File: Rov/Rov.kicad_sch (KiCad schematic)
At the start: 1 part, among them Q1 IRLZ44N

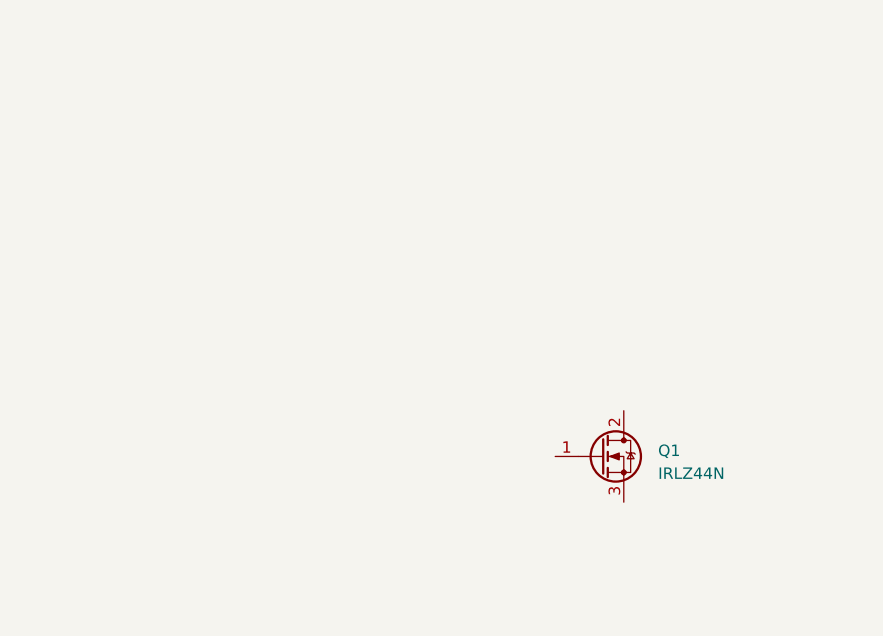
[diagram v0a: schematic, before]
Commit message: Learning kicad
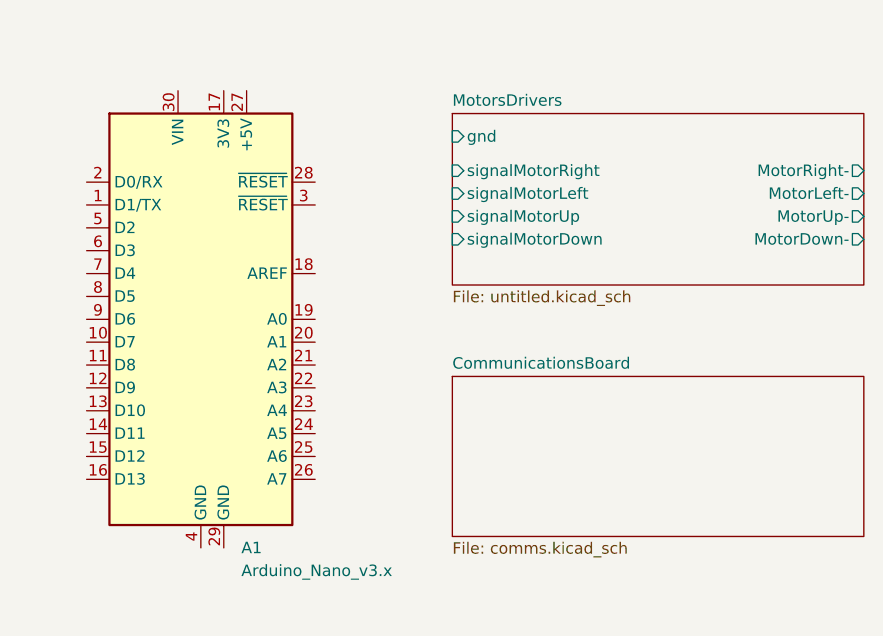
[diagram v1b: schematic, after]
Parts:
- removed Q1: IRLZ44N, Package_TO_SOT_THT:TO-220-3_Vertical, symbol Transistor_FET:IRLZ44N
- added A1: Arduino_Nano_v3.x, Module:Arduino_Nano, symbol MCU_Module:Arduino_Nano_v3.x
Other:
- added sheet CommunicationsBoard (comms.kicad_sch)
- added sheet MotorsDrivers (untitled.kicad_sch)
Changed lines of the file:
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@@
 (kicad_sch (version 20230121) (generator eeschema)
   (paper "A4")
-  (symbol (lib_id "Transistor_FET:IRLZ44N") (at 120.65 90.17 0) (unit 1)
+  (symbol (lib_id "MCU_Module:Arduino_Nano_v3.x") (at 76.2 74.93 0) (unit 1)
     (in_bom yes) (on_board yes) (dnp no) (fields_autoplaced)
-    (property "Reference" "Q1" (at 127 89.535 0)
+    (property "Reference" "A1" (at 80.6959 100.33 0)
       (effects (font (size 1.27 1.27)) (justify left))
     )
-    (property "Value" "IRLZ44N" (at 127 92.075 0)
+    (property "Value" "Arduino_Nano_v3.x" (at 80.6959 102.87 0)
       (effects (font (size 1.27 1.27)) (justify left))
     )
-    (property "Footprint" "Package_TO_SOT_THT:TO-220-3_Vertical" (at 127 92.075 0)
-      (effects (font (size 1.27 1.27) italic) (justify left) hide)
+    (property "Footprint" "Module:Arduino_Nano" (at 76.2 74.93 0)
+      (effects (font (size 1.27 1.27) italic) hide)
     )
-    (property "Datasheet" "http://www.irf.com/product-info/datasheets/data/irlz44n.pdf" (at 120.65 90.17 0)
-      (effects (font (size 1.27 1.27)) (justify left) hide)
+    (property "Datasheet" "http://www.mouser.com/pdfdocs/Gravitech_Arduino_Nano3_0.pdf" (at 76.2 74.93 0)
+      (effects (font (size 1.27 1.27)) hide)
     )
     (pin "1")
+    (pin "10")
+    (pin "11")
+    (pin "12")
+    (pin "13")
+    (pin "14")
+    (pin "15")
+    (pin "16")
+    (pin "17")
+    (pin "18")
+    (pin "19")
     (pin "2")
+    (pin "20")
+    (pin "21")
+    (pin "22")
+    (pin "23")
+    (pin "24")
+    (pin "25")
+    (pin "26")
+    (pin "27")
+    (pin "28")
+    (pin "29")
     (pin "3")
+    (pin "30")
+    (pin "4")
+    (pin "5")
+    (pin "6")
+    (pin "7")
+    (pin "8")
+    (pin "9")
     (instances
       (project "Rov"
         (path "/195799e7-2545-43ed-8a08-3008b09b45b7"
-          (reference "Q1") (unit 1)
+          (reference "A1") (unit 1)
         )
       )
     )
+  )
+  (sheet (at 104.14 81.28) (size 45.72 17.78) (fields_autoplaced)
+    (stroke (width 0.1524) (type solid))
+    (fill (color 0 0 0 0.0000))
+    (property "Sheetname" "CommunicationsBoard" (at 104.14 80.5684 0)
+      (effects (font (size 1.27 1.27)) (justify left bottom))
+    )
+    (property "Sheetfile" "comms.kicad_sch" (at 104.14 99.6446 0)
+      (effects (font (size 1.27 1.27)) (justify left top))
+    )
+    (instances
+      (project "Rov"
+        (path "/195799e7-2545-43ed-8a08-3008b09b45b7" (page "3"))
+      )
+    )
+  )
+  (sheet (at 104.14 52.07) (size 45.72 19.05) (fields_autoplaced)
+    (stroke (width 0.1524) (type solid))
+    (fill (color 0 0 0 0.0000))
+    (property "Sheetname" "MotorsDrivers" (at 104.14 51.3584 0)
+      (effects (font (size 1.27 1.27)) (justify left bottom))
+    )
+    (property "Sheetfile" "untitled.kicad_sch" (at 104.14 71.7046 0)
+      (effects (font (size 1.27 1.27)) (justify left top))
+    )
+    (pin "MotorRight-" output (at 149.86 58.42 0)
+      (effects (font (size 1.27 1.27)) (justify right))
+    )
+    (pin "MotorDown-" output (at 149.86 66.04 0)
+      (effects (font (size 1.27 1.27)) (justify right))
+    )
+    (pin "MotorUp-" output (at 149.86 63.5 0)
+      (effects (font (size 1.27 1.27)) (justify right))
+    )
+    (pin "MotorLeft-" output (at 149.86 60.96 0)
+      (effects (font (size 1.27 1.27)) (justify right))
+    )
+    (pin "gnd" input (at 104.14 54.61 180)
+      (effects (font (size 1.27 1.27)) (justify left))
+    )
+    (pin "signalMotorRight" input (at 104.14 58.42 180)
+      (effects (font (size 1.27 1.27)) (justify left))
+    )
+    (pin "signalMotorLeft" input (at 104.14 60.96 180)
+      (effects (font (size 1.27 1.27)) (justify left))
+    )
+    (pin "signalMotorUp" input (at 104.14 63.5 180)
+      (effects (font (size 1.27 1.27)) (justify left))
+    )
+    (pin "signalMotorDown" input (at 104.14 66.04 180)
+      (effects (font (size 1.27 1.27)) (justify left))
+    )
+    (instances
+      (project "Rov"
+        (path "/195799e7-2545-43ed-8a08-3008b09b45b7" (page "2"))
+      )
+    )

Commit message: Added more wiring
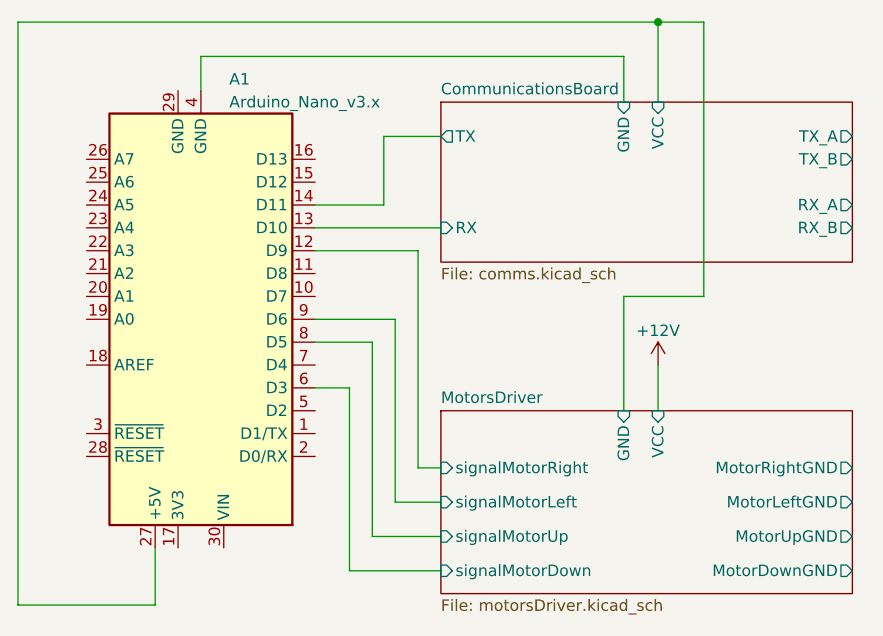
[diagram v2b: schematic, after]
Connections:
- net MotorsDriver/signalMotorRight: now reaches A1.12 (D9)
- net CommunicationsBoard/RX: now reaches A1.13 (D10)
- net CommunicationsBoard/TX: now reaches A1.14 (D11)
- net CommunicationsBoard/VCC: now reaches A1.27 (+5V)
- net CommunicationsBoard/GND: now reaches A1.4 (GND)
- net MotorsDriver/signalMotorDown: now reaches A1.6 (D3)
- net MotorsDriver/signalMotorUp: now reaches A1.8 (D5)
- net MotorsDriver/signalMotorLeft: now reaches A1.9 (D6)
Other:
- removed sheet MotorsDrivers
- added sheet MotorsDriver (motorsDriver.kicad_sch)
- sheet CommunicationsBoard ports: added GND, RX, RX_A, RX_B, TX, TX_A, TX_B, VCC; removed none
- moved on the sheet: A1
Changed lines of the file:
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@@
 (kicad_sch (version 20230121) (generator eeschema)
   (paper "A4")
-  (symbol (lib_id "MCU_Module:Arduino_Nano_v3.x") (at 76.2 74.93 0) (unit 1)
+  (junction (at 127 41.91) (diameter 0) (color 0 0 0 0)
+  )
+  (wire (pts (xy 95.25 99.06) (xy 95.25 77.47))
+    (stroke (width 0) (type default))
+  )
+  (wire (pts (xy 96.52 54.61) (xy 102.87 54.61))
+    (stroke (width 0) (type default))
+  )
+  (wire (pts (xy 102.87 91.44) (xy 100.33 91.44))
+    (stroke (width 0) (type default))
+  )
+  (wire (pts (xy 132.08 72.39) (xy 132.08 41.91))
+    (stroke (width 0) (type default))
+  )
+  (wire (pts (xy 76.2 45.72) (xy 123.19 45.72))
+    (stroke (width 0) (type default))
+  )
+  (wire (pts (xy 96.52 54.61) (xy 96.52 62.23))
+    (stroke (width 0) (type default))
+  )
+  (wire (pts (xy 97.79 95.25) (xy 102.87 95.25))
+    (stroke (width 0) (type default))
+  )
+  (wire (pts (xy 55.88 41.91) (xy 55.88 106.68))
+    (stroke (width 0) (type default))
+  )
+  (wire (pts (xy 132.08 41.91) (xy 127 41.91))
+    (stroke (width 0) (type default))
+  )
+  (wire (pts (xy 92.71 102.87) (xy 102.87 102.87))
+    (stroke (width 0) (type default))
+  )
+  (wire (pts (xy 123.19 45.72) (xy 123.19 50.8))
+    (stroke (width 0) (type default))
+  )
+  (wire (pts (xy 76.2 49.53) (xy 76.2 45.72))
+    (stroke (width 0) (type default))
+  )
+  (wire (pts (xy 123.19 85.09) (xy 123.19 72.39))
+    (stroke (width 0) (type default))
+  )
+  (wire (pts (xy 127 41.91) (xy 55.88 41.91))
+    (stroke (width 0) (type default))
+  )
+  (wire (pts (xy 100.33 67.31) (xy 88.9 67.31))
+    (stroke (width 0) (type default))
+  )
+  (wire (pts (xy 92.71 82.55) (xy 92.71 102.87))
+    (stroke (width 0) (type default))
+  )
+  (wire (pts (xy 88.9 74.93) (xy 97.79 74.93))
+    (stroke (width 0) (type default))
+  )
+  (wire (pts (xy 88.9 82.55) (xy 92.71 82.55))
+    (stroke (width 0) (type default))
+  )
+  (wire (pts (xy 88.9 77.47) (xy 95.25 77.47))
+    (stroke (width 0) (type default))
+  )
+  (wire (pts (xy 127 50.8) (xy 127 41.91))
+    (stroke (width 0) (type default))
+  )
+  (wire (pts (xy 88.9 62.23) (xy 96.52 62.23))
+    (stroke (width 0) (type default))
+  )
+  (wire (pts (xy 102.87 99.06) (xy 95.25 99.06))
+    (stroke (width 0) (type default))
+  )
+  (wire (pts (xy 127 80.01) (xy 127 85.09))
+    (stroke (width 0) (type default))
+  )
+  (wire (pts (xy 71.12 106.68) (xy 71.12 100.33))
+    (stroke (width 0) (type default))
+  )
+  (wire (pts (xy 55.88 106.68) (xy 71.12 106.68))
+    (stroke (width 0) (type default))
+  )
+  (wire (pts (xy 88.9 64.77) (xy 102.87 64.77))
+    (stroke (width 0) (type default))
+  )
+  (wire (pts (xy 97.79 74.93) (xy 97.79 95.25))
+    (stroke (width 0) (type default))
+  )
+  (wire (pts (xy 100.33 91.44) (xy 100.33 67.31))
+    (stroke (width 0) (type default))
+  )
+  (wire (pts (xy 123.19 72.39) (xy 132.08 72.39))
+    (stroke (width 0) (type default))
+  )
+  (symbol (lib_id "power:+12V") (at 127 80.01 0) (unit 1)
     (in_bom yes) (on_board yes) (dnp no) (fields_autoplaced)
-    (property "Reference" "A1" (at 80.6959 100.33 0)
-      (effects (font (size 1.27 1.27)) (justify left))
-    )
-    (property "Value" "Arduino_Nano_v3.x" (at 80.6959 102.87 0)
-      (effects (font (size 1.27 1.27)) (justify left))
+    (property "Reference" "#PWR01" (at 127 83.82 0)
+      (effects (font (size 1.27 1.27)) hide)
+    )
+    (property "Value" "+12V" (at 127 76.2 0)
+      (effects (font (size 1.27 1.27)))
+    )
+    (property "Footprint" "" (at 127 80.01 0)
+      (effects (font (size 1.27 1.27)) hide)
+    )
+    (property "Datasheet" "" (at 127 80.01 0)
+      (effects (font (size 1.27 1.27)) hide)
+    )
+    (pin "1")
+    (instances
+      (project "Rov"
+        (path "/195799e7-2545-43ed-8a08-3008b09b45b7"
+          (reference "#PWR01") (unit 1)
+        )
+      )
+    )
+  )
+  (symbol (lib_id "MCU_Module:Arduino_Nano_v3.x") (at 76.2 74.93 180) (unit 1)
+    (in_bom yes) (on_board yes) (dnp no) (fields_autoplaced)
+    (property "Reference" "A1" (at 79.3497 48.26 0)
+      (effects (font (size 1.27 1.27)) (justify right))
+    )
+    (property "Value" "Arduino_Nano_v3.x" (at 79.3497 50.8 0)
+      (effects (font (size 1.27 1.27)) (justify right))
     )
     (property "Footprint" "Module:Arduino_Nano" (at 76.2 74.93 0)
@@
     )
   )
-  (sheet (at 104.14 81.28) (size 45.72 17.78) (fields_autoplaced)
+  (sheet (at 102.87 50.8) (size 45.72 17.78) (fields_autoplaced)
     (stroke (width 0.1524) (type solid))
     (fill (color 0 0 0 0.0000))
-    (property "Sheetname" "CommunicationsBoard" (at 104.14 80.5684 0)
+    (property "Sheetname" "CommunicationsBoard" (at 102.87 50.0884 0)
       (effects (font (size 1.27 1.27)) (justify left bottom))
     )
-    (property "Sheetfile" "comms.kicad_sch" (at 104.14 99.6446 0)
+    (property "Sheetfile" "comms.kicad_sch" (at 102.87 69.1646 0)
       (effects (font (size 1.27 1.27)) (justify left top))
     )
+    (pin "TX_B" output (at 148.59 57.15 0)
+      (effects (font (size 1.27 1.27)) (justify right))
+    )
+    (pin "TX_A" output (at 148.59 54.61 0)
+      (effects (font (size 1.27 1.27)) (justify right))
+    )
+    (pin "RX_B" output (at 148.59 64.77 0)
+      (effects (font (size 1.27 1.27)) (justify right))
+    )
+    (pin "RX_A" output (at 148.59 62.23 0)
+      (effects (font (size 1.27 1.27)) (justify right))
+    )
+    (pin "VCC" input (at 127 50.8 90)
+      (effects (font (size 1.27 1.27)) (justify right))
+    )
+    (pin "GND" input (at 123.19 50.8 90)
+      (effects (font (size 1.27 1.27)) (justify right))
+    )
+    (pin "RX" input (at 102.87 64.77 180)
+      (effects (font (size 1.27 1.27)) (justify left))
+    )
+    (pin "TX" output (at 102.87 54.61 180)
+      (effects (font (size 1.27 1.27)) (justify left))
+    )
     (instances
       (project "Rov"
@@
     )
   )
-  (sheet (at 104.14 52.07) (size 45.72 19.05) (fields_autoplaced)
+  (sheet (at 102.87 85.09) (size 45.72 20.32) (fields_autoplaced)
     (stroke (width 0.1524) (type solid))
     (fill (color 0 0 0 0.0000))
-    (property "Sheetname" "MotorsDrivers" (at 104.14 51.3584 0)
+    (property "Sheetname" "MotorsDriver" (at 102.87 84.3784 0)
       (effects (font (size 1.27 1.27)) (justify left bottom))
     )
-    (property "Sheetfile" "untitled.kicad_sch" (at 104.14 71.7046 0)
+    (property "Sheetfile" "motorsDriver.kicad_sch" (at 102.87 105.9946 0)
       (effects (font (size 1.27 1.27)) (justify left top))
     )
-    (pin "MotorRight-" output (at 149.86 58.42 0)
-      (effects (font (size 1.27 1.27)) (justify right))
-    )
-    (pin "MotorDown-" output (at 149.86 66.04 0)
-      (effects (font (size 1.27 1.27)) (justify right))
-    )
-    (pin "MotorUp-" output (at 149.86 63.5 0)
-      (effects (font (size 1.27 1.27)) (justify right))
-    )
-    (pin "MotorLeft-" output (at 149.86 60.96 0)
-      (effects (font (size 1.27 1.27)) (justify right))
-    )
-    (pin "gnd" input (at 104.14 54.61 180)
-      (effects (font (size 1.27 1.27)) (justify left))
-    )
-    (pin "signalMotorRight" input (at 104.14 58.42 180)
-      (effects (font (size 1.27 1.27)) (justify left))
-    )
-    (pin "signalMotorLeft" input (at 104.14 60.96 180)
-      (effects (font (size 1.27 1.27)) (justify left))
-    )
-    (pin "signalMotorUp" input (at 104.14 63.5 180)
-      (effects (font (size 1.27 1.27)) (justify left))
-    )
-    (pin "signalMotorDown" input (at 104.14 66.04 180)
-      (effects (font (size 1.27 1.27)) (justify left))
-    )
-    (instances
-      (project "Rov"
-        (path "/195799e7-2545-43ed-8a08-3008b09b45b7" (page "2"))
-      )
-    )
+    (pin "MotorUpGND" output (at 148.59 99.06 0)
+      (effects (font (size 1.27 1.27)) (justify right))
+    )
+    (pin "MotorLeftGND" output (at 148.59 95.25 0)
+      (effects (font (size 1.27 1.27)) (justify right))
+    )
+    (pin "MotorRightGND" output (at 148.59 91.44 0)
+      (effects (font (size 1.27 1.27)) (justify right))
+    )
+    (pin "MotorDownGND" output (at 148.59 102.87 0)
+      (effects (font (size 1.27 1.27)) (justify right))
+    )
+    (pin "signalMotorLeft" input (at 102.87 95.25 180)
+      (effects (font (size 1.27 1.27)) (justify left))
+    )
+    (pin "GND" input (at 123.19 85.09 90)
+      (effects (font (size 1.27 1.27)) (justify right))
+    )
+    (pin "signalMotorUp" input (at 102.87 99.06 180)
+      (effects (font (size 1.27 1.27)) (justify left))
+    )
+    (pin "signalMotorRight" input (at 102.87 91.44 180)
+      (effects (font (size 1.27 1.27)) (justify left))
+    )
+    (pin "signalMotorDown" input (at 102.87 102.87 180)
+      (effects (font (size 1.27 1.27)) (justify left))
+    )
+    (pin "VCC" input (at 127 85.09 90)
+      (effects (font (size 1.27 1.27)) (justify right))
+    )
+    (instances
+      (project "Rov"
+        (path "/195799e7-2545-43ed-8a08-3008b09b45b7" (page "3"))
+      )
+    )
